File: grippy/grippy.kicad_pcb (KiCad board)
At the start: 2 copper layers, 66.1 x 35.4 mm, 9 parts, among them J1 Conn_01x08_Socket, SW0 SW_SPST, SW1 SW_SPST, SW2 SW_SPST, SW3 SW_SPST, SW4 SW_SPST, SW5 SW_DPDT_x2, U1 esp32s3-supermini

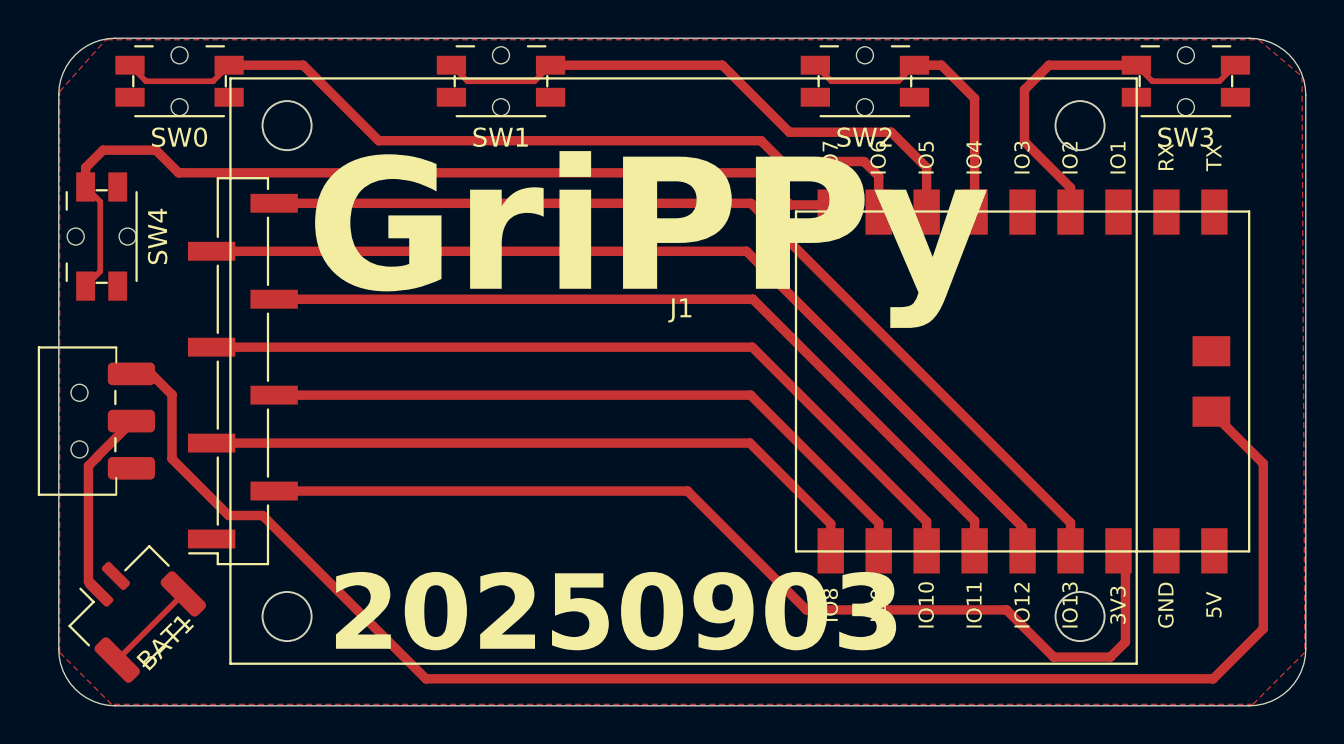
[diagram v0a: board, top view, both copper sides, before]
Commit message: got a fairly usable case
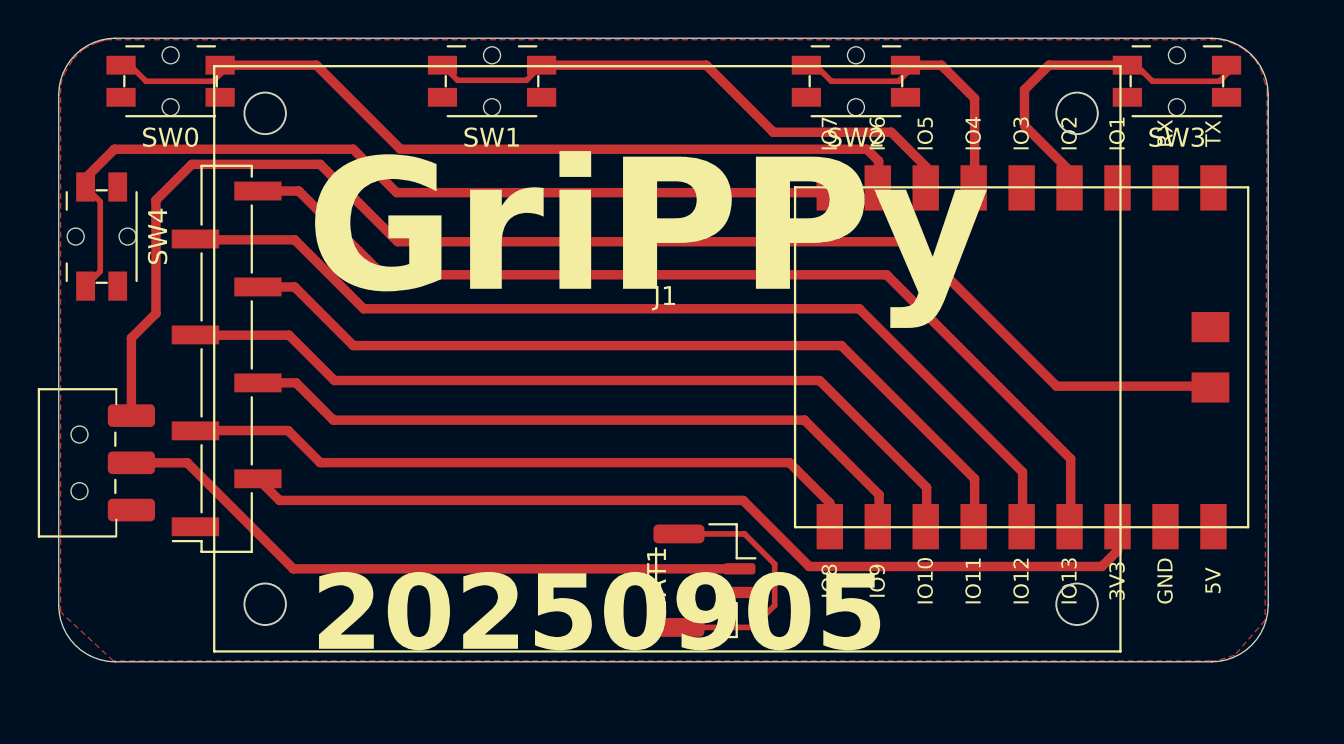
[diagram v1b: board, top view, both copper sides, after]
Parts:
- moved BAT1 30.3 mm to (207.4, 97.2), turned to -90 degrees
- moved SW5 2.21 mm to (174.6, 91.0)
- moved U1 1.28 mm to (224.2, 85.4)
- moved J1 1.08 mm to (205.4, 85.5)
- moved SW0 0.47 mm to (179.1, 70.8)
- moved SW1 0.47 mm to (196.2, 70.8)
- moved SW2 0.47 mm to (215.4, 70.8)
- moved SW3 0.47 mm to (232.4, 70.8)
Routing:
- net /B+: track 10.3 -> 34.5 mm
- net /mp: track 4.95 -> 13.5 mm
- net /RAW: track 82.4 -> 73.9 mm
- net VCC: track 54.0 -> 49.1 mm
- net /BLK: track 50.7 -> 52.5 mm
- net /DC: track 43.5 -> 44.6 mm
- net /pinky: track 19.9 -> 18.9 mm
- net /ring: track 15.9 -> 14.9 mm
- net /CS: track 50.3 -> 51.0 mm
- net /thumb: track 48.1 -> 47.4 mm
- net /SDA: track 36.3 -> 37.0 mm
- net /middle: track 30.5 -> 29.9 mm
- net /index: track 44.7 -> 44.2 mm
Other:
- board size 66.1 x 35.4 mm -> 64.1 x 33 mm
- board text added: "20250905"
- board text removed: "20250903"
